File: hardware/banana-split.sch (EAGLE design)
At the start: 45 parts, among them IC1 REG1117, IC2 4050D, IC3 PIC12F1822SO08, IC4 6N138, X1 DIN5PIN, X2 DIN5PIN, X3 DIN5PIN, X4 DIN5PIN, X5 DIN5PIN, X6 DIN5PIN, X7 VERTICAL_3_5MM_SOCKET

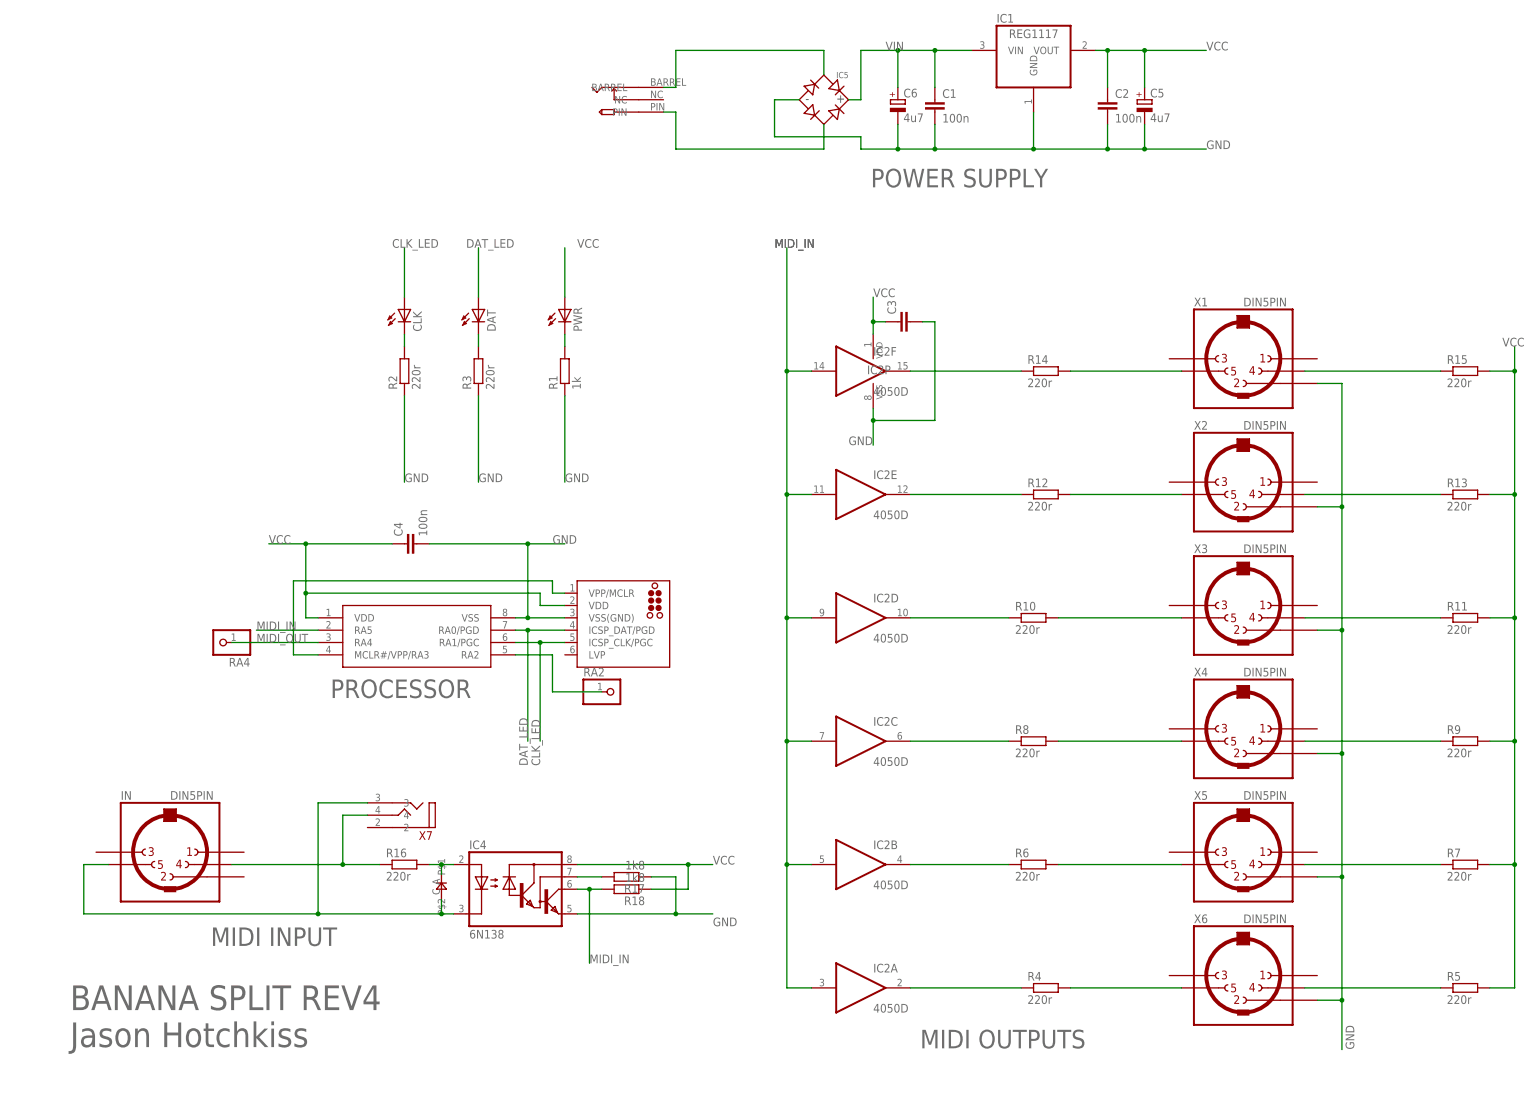
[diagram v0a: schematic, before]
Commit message: V5 PCB
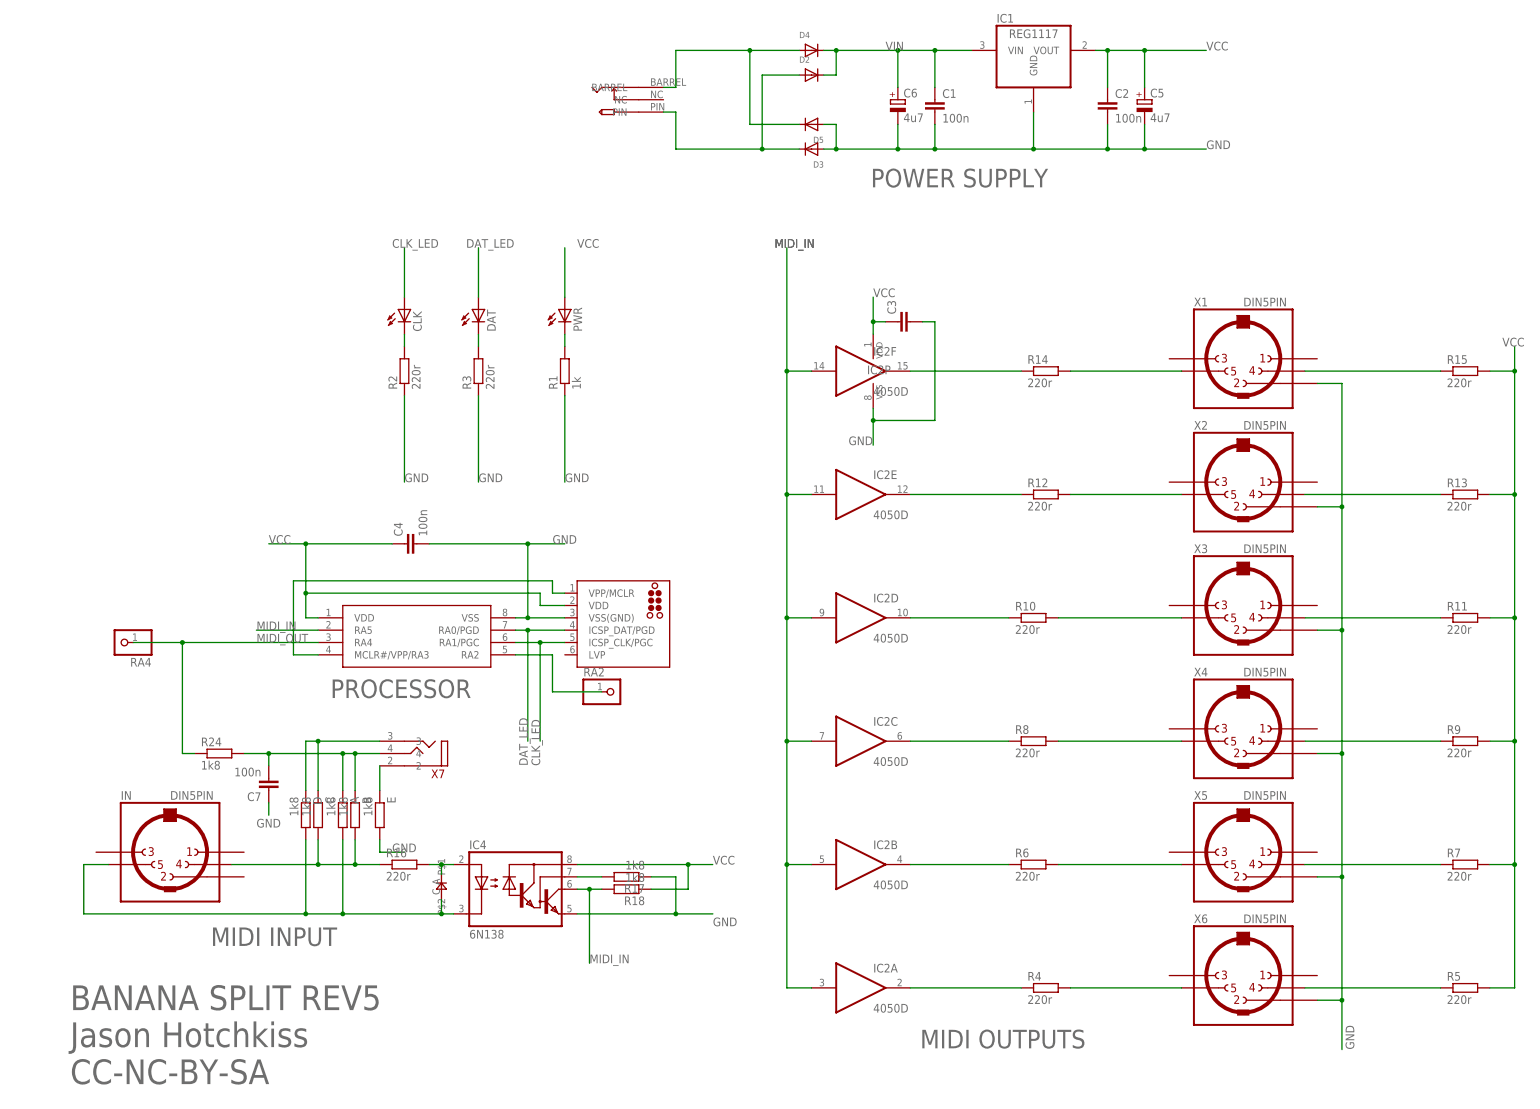
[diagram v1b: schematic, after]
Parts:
- removed IC5: (no value), microbuilder:BRIDGERECTIFIER
- added A, B, C, D, E: 1k8, rcl:R-EU_R0603
- added C7: 100n, rcl:C-EUC0805
- added D2, D3, D4, D5: (no value), adafruit:DIODESOD-123
- added R24: 1k8, rcl:R-EU_R0805
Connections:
- new net N$26: C.1, D.1, X7.3
- new net N$29: E.1, X7.2
- new net N$30: A.1, B.1, C7.2, R24.2, X7.4
- net GND: now also C7.1, D3.A, D5.A, E.2; no longer IC5.-
- net MIDI_OUT: now also R24.1
- net N$20: now also B.2, C.2; no longer X7.4
- net N$24: now also A.2, D.2; no longer X7.3
- net N$27: now also D4.A, D5.C; no longer IC5.AC1
- net N$28: now also D2.A, D3.C; no longer IC5.AC2
- net VIN: now also D2.C, D4.C; no longer IC5.+
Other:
- note added: "BANANA SPLIT REV5"
- note added: "Jason Hotchkiss CC-NC-BY-SA"
- note removed: "BANANA SPLIT REV4"
- note removed: "Jason Hotchkiss"
- moved on the sheet: RA4, X7

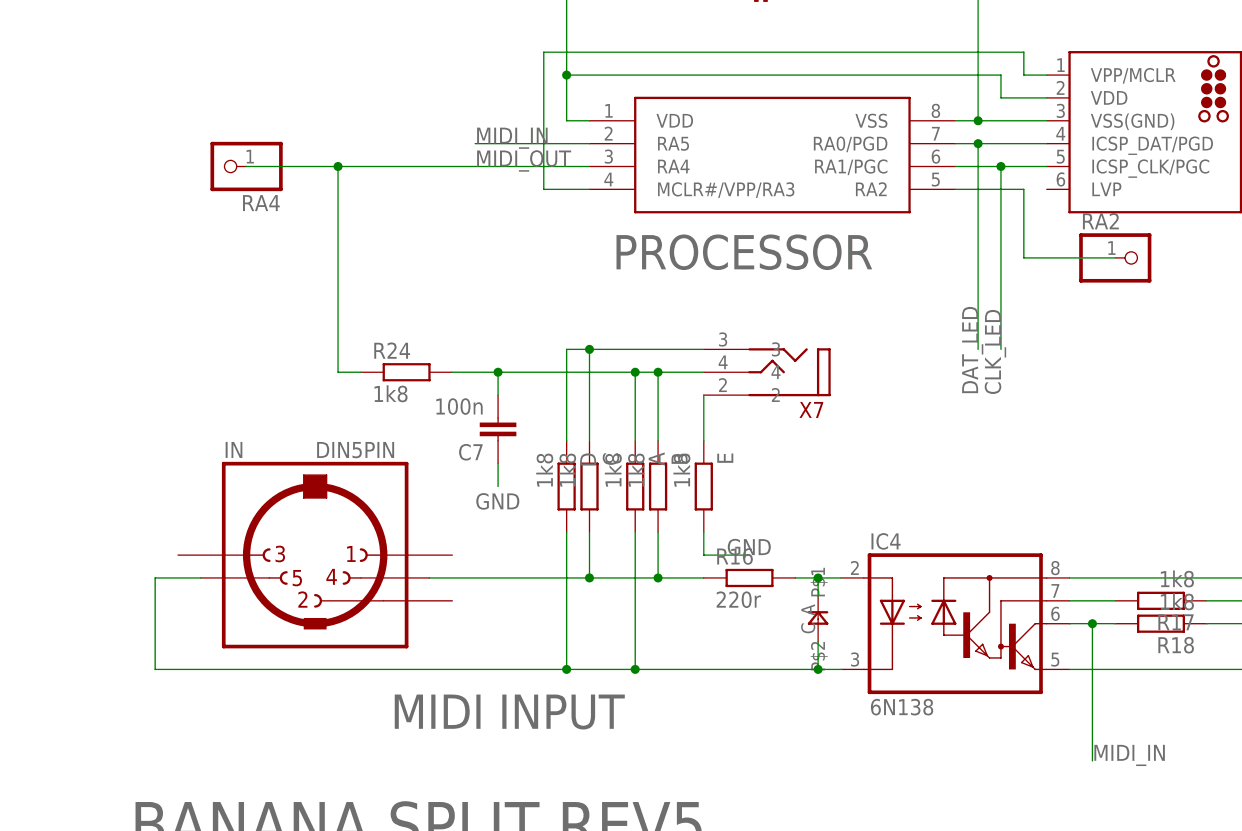
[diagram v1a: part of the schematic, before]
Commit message: v6 candidate
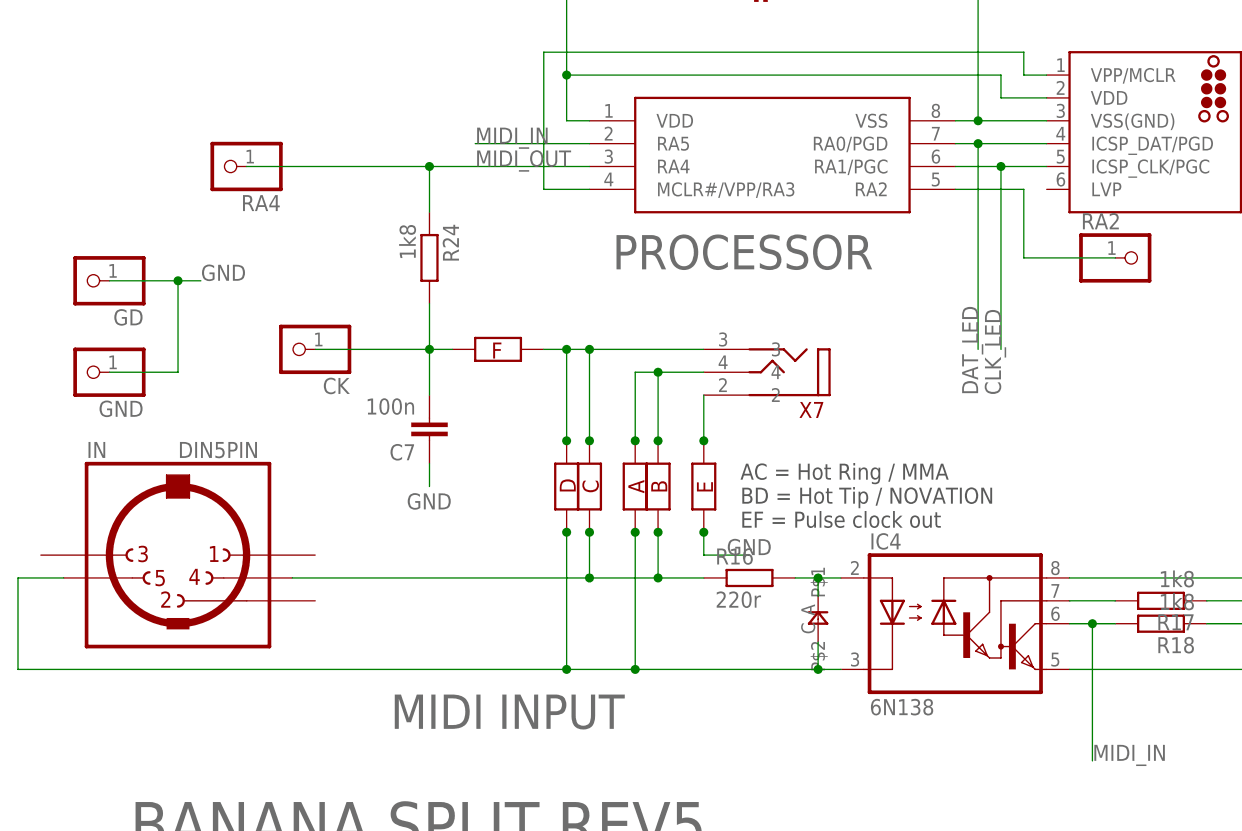
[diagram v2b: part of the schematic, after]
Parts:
- added CK, GD, GND: (no value), pinhead:PINHD-1X1
- added F: JH_JP, jason_eagle6:JH_JP
- A, B, C, D, E: value 1k8 -> JH_JP; device rcl:R-EU_R0603 -> jason_eagle6:JH_JP
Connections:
- new net N$31: C7.2, CK.1, F.P$1, R24.2
- net GND: now also E.P$1, GD.1, GND.1; no longer E.2
- net N$20: now also B.P$1, C.P$1; no longer B.2, C.2
- net N$24: now also A.P$1, D.P$1; no longer A.2, D.2
- net N$26: now also C.P$2, D.P$2, F.P$2; no longer C.1, D.1
- net N$29: now also E.P$2; no longer E.1
- net N$30: now also A.P$2, B.P$2; no longer A.1, B.1, C7.2, R24.2
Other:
- note added: "AC = Hot Ring / MMA BD = Hot Tip / NOVATION EF = Pulse clock out"
- moved on the sheet: A, B, C, C7, D, E, IN, R24

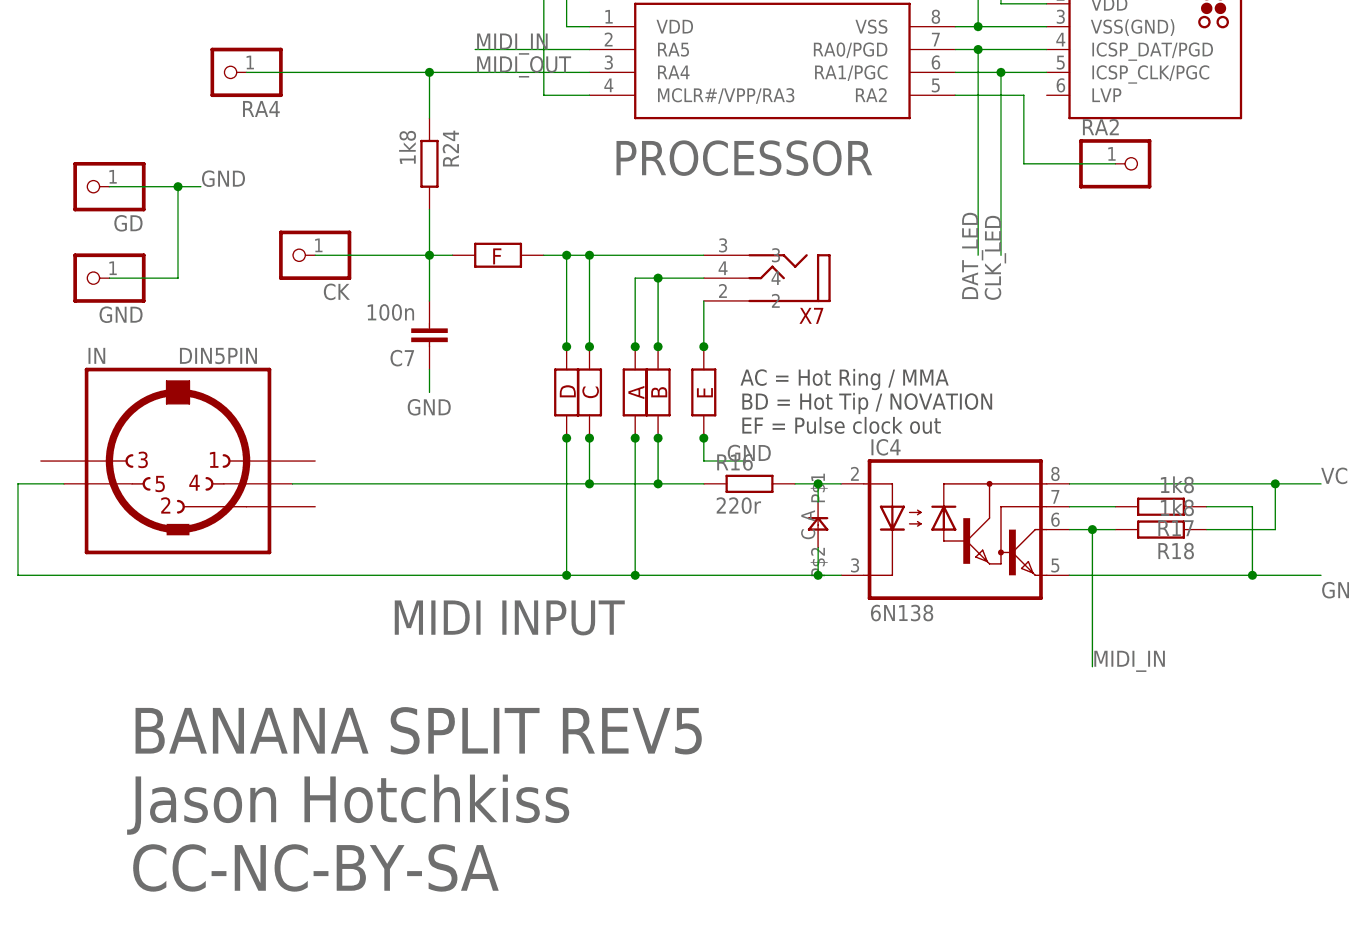
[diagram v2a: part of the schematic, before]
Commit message: V7 PCB
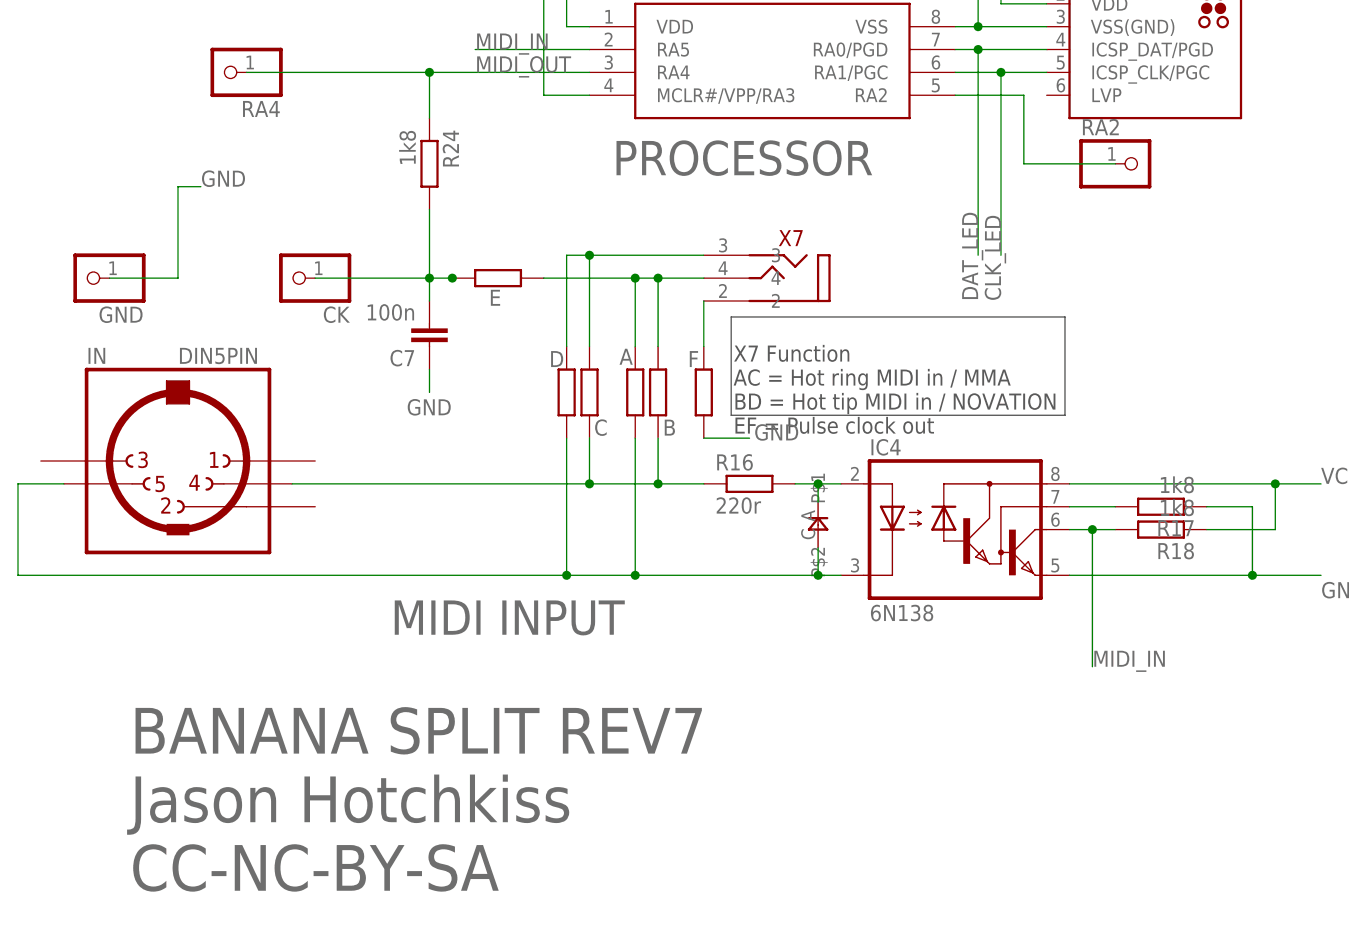
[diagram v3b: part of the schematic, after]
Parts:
- removed GD: (no value), pinhead:PINHD-1X1
- A, B, C, D, E, F: value JH_JP -> 1k8; device jason_eagle6:JH_JP -> rcl:R-EU_R0805
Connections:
- net GND: now also F.1; no longer E.P$1, GD.1
- net N$20: now also B.1, C.1; no longer B.P$1, C.P$1
- net N$24: now also A.1, D.1; no longer A.P$1, D.P$1
- net N$26: now also C.2, D.2; no longer C.P$2, D.P$2, F.P$2
- net N$29: now also F.2; no longer E.P$2
- net N$30: now also A.2, B.2, E.2; no longer A.P$2, B.P$2
- net N$31: now also E.1; no longer F.P$1
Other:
- note added: "BANANA SPLIT REV7"
- note added: "X7 Function AC = Hot ring MIDI in / MMA BD = Hot tip MIDI in / NOVATION EF = Pulse clock out"
- note removed: "AC = Hot Ring / MMA BD = Hot Tip / NOVATION EF = Pulse clock out"
- note removed: "BANANA SPLIT REV5"
- moved on the sheet: CK, E, F
